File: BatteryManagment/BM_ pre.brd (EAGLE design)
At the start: 107.7 x 100 mm, 123 parts, among them IC1 LMV321M5, U1 ATMEGA328P-AU, U2 LTC4440EMS8E-5PBF

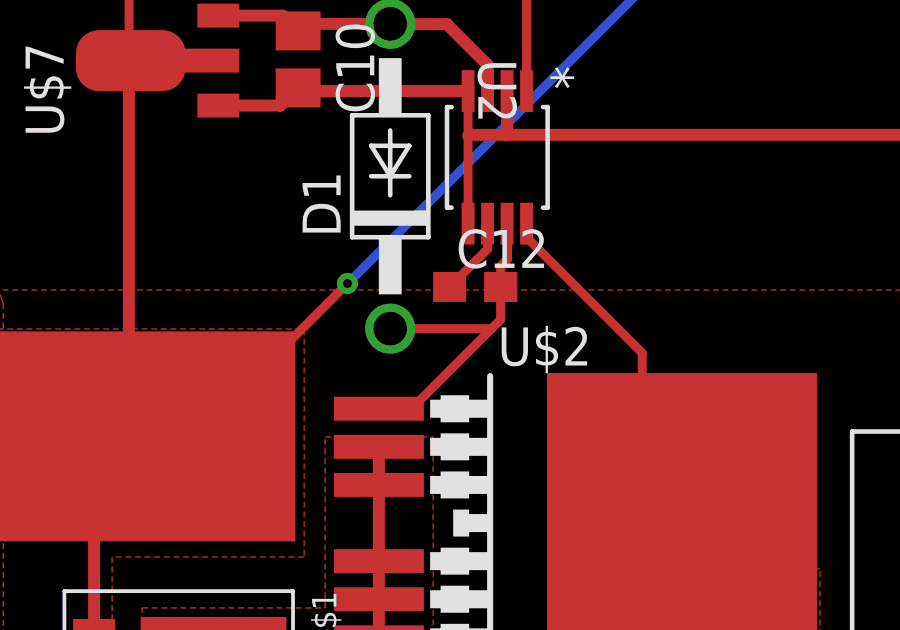
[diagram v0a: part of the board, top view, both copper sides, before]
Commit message: Revert "Revert "Finished version v0.2""
This reverts commit 5ce350199b8ee6846b212b42396474e627ee3767.
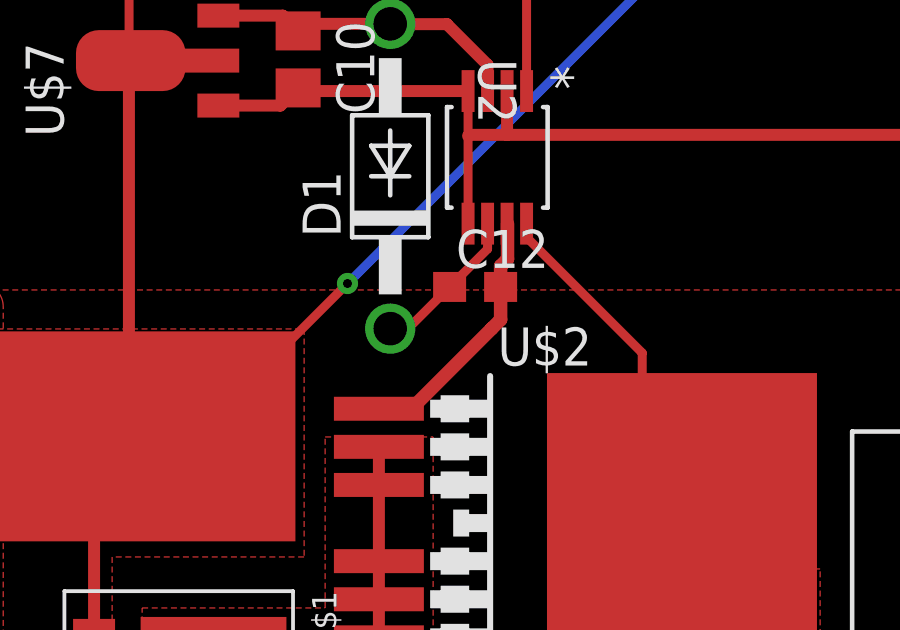
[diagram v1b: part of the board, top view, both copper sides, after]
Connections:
- net CHARGE_CONTROL: no longer D1.C
- net N$2: now also D1.C
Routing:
- net CHARGE_CONTROL: track 12.0 -> 8.60 mm
- net N$2: track 2.63 -> 5.19 mm
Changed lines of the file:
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@@
 <signal name="CHARGE_CONTROL">
 <contactref element="U$2" pad="1"/>
+<wire x1="22.25" y1="30.31" x2="19.66" y2="27.72" width="0.45" layer="1"/>
+<wire x1="19.66" y1="27.72" x2="18.5725" y2="27.72" width="0.3" layer="1"/>
+<wire x1="18.5725" y1="27.72" x2="18.4925" y2="27.64" width="0.3" layer="1"/>
+<wire x1="22.55" y1="30.61" x2="22.25" y2="30.31" width="0.45" layer="1"/>
 <contactref element="U2" pad="7"/>
 <contactref element="C12" pad="2"/>
-<contactref element="D1" pad="C"/>
 <wire x1="22.765" y1="33.8102" x2="22.78" y2="33.8102" width="0.3" layer="1"/>
-<wire x1="22.78" y1="32.63" x2="22.55" y2="32.4" width="0.3" layer="1"/>
-<wire x1="22.55" y1="32.4" x2="22.55" y2="31.7" width="0.3" layer="1"/>
-<wire x1="22.78" y1="33.8102" x2="22.78" y2="32.63" width="0.3" layer="1"/>
-<wire x1="22.55" y1="30.61" x2="22.55" y2="31.7" width="0.3" layer="1"/>
-<wire x1="22.25" y1="30.31" x2="19.66" y2="27.72" width="0.3" layer="1"/>
-<wire x1="19.66" y1="27.72" x2="18.5725" y2="27.72" width="0.3" layer="1"/>
-<wire x1="18.5725" y1="27.72" x2="18.4925" y2="27.64" width="0.3" layer="1"/>
-<wire x1="18.87" y1="30.31" x2="22.25" y2="30.31" width="0.3" layer="1"/>
-<wire x1="22.25" y1="30.31" x2="22.55" y2="30.61" width="0.3" layer="1"/>
+<wire x1="22.78" y1="32.63" x2="22.55" y2="32.4" width="0.45" layer="1"/>
+<wire x1="22.55" y1="32.4" x2="22.55" y2="31.7" width="0.45" layer="1"/>
+<wire x1="22.78" y1="33.8102" x2="22.78" y2="32.63" width="0.45" layer="1"/>
+<wire x1="22.55" y1="31.7" x2="22.55" y2="30.61" width="0.45" layer="1"/>
 </signal>
 <signal name="MOTOR_CONTROL">
@@
 <wire x1="22.115" y1="33.8102" x2="22.115" y2="32.965" width="0.3" layer="1"/>
 <wire x1="22.115" y1="32.965" x2="20.85" y2="31.7" width="0.3" layer="1"/>
+<contactref element="D1" pad="C"/>
+<wire x1="20.85" y1="31.7" x2="19.46" y2="30.31" width="0.3" layer="1"/>
+<wire x1="19.46" y1="30.31" x2="18.87" y2="30.31" width="0.3" layer="1"/>
 </signal>
 <signal name="N$17">
